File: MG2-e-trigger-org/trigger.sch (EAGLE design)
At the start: 20 parts, among them IC1 4538D, T1 BC847, T2 BC847

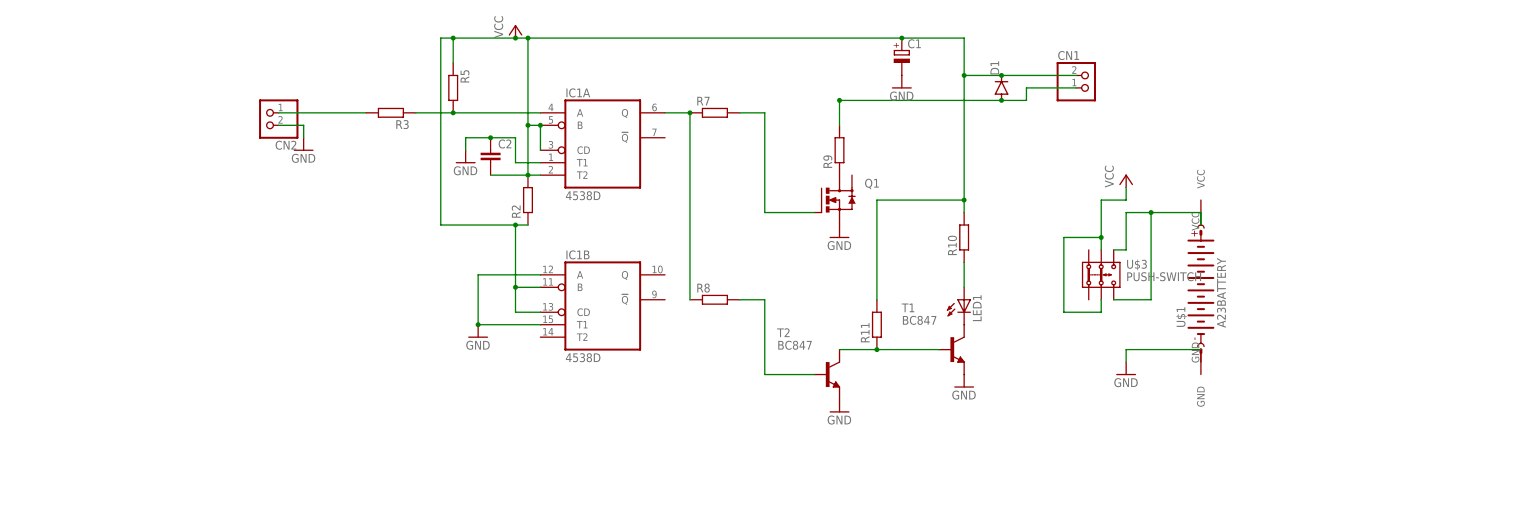
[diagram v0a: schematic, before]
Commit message: MG2 trigger
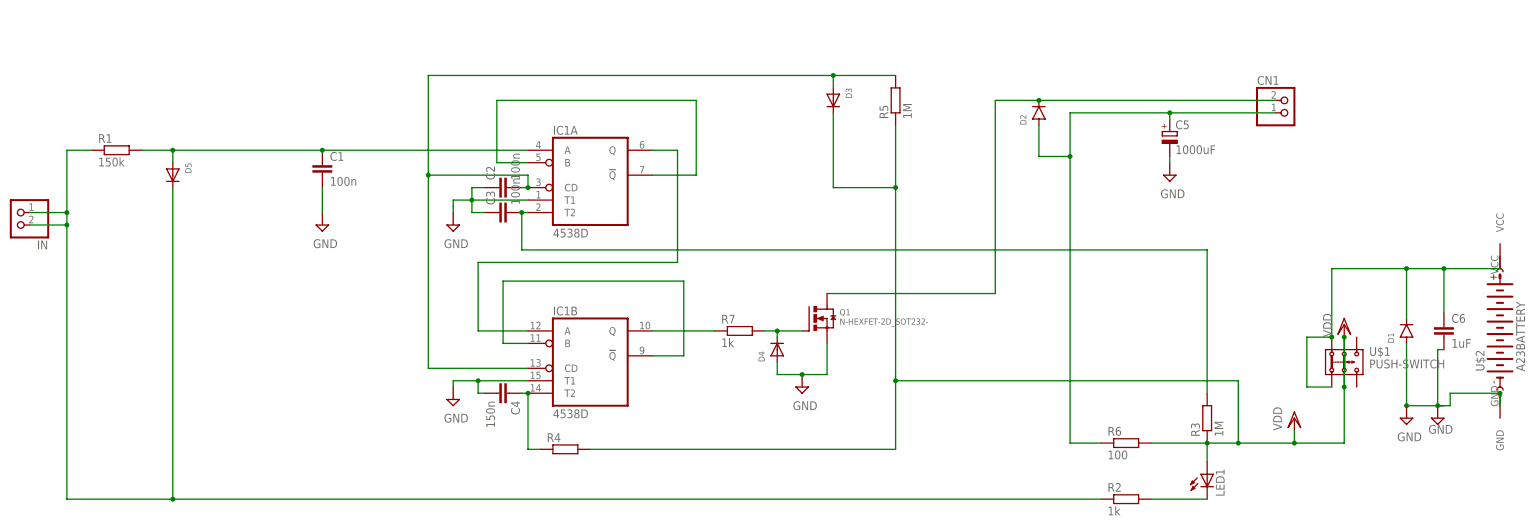
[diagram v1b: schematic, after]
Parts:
- removed CN2: (no value), adafruit:JST_2PIN-THM
- removed R10, R11: (no value), eagle-ltspice:R
- removed R8, R9: (no value), eagle-ltspice:RR1206
- removed T1, T2: BC847, nxp_60:BC847
- removed U$3: PUSH-SWITCH, zort-library:PUSH-SWITCH
- added C3: 100n, eagle-ltspice:C
- added C4: 150n, eagle-ltspice:C
- added C5: 1000uF, rcl:CPOL-EUE5-6
- added C6: 1uF, eagle-ltspice:CC1808
- added D2: (no value), semicon-smd-ipc:D-SMB
- added D3, D4, D5: (no value), adafruit:DIODESOD-123
- added IN: (no value), adafruit:JST_2PIN-THM
- added R1: 150k, eagle-ltspice:RR1206
- added R4: (no value), eagle-ltspice:RR1206
- added R6: 100, eagle-ltspice:RR2512
- added U$2: A23BATTERY, zort-library:A23BATTERY
- C1: value (none) -> 100n; device rcl:CPOL-EUE5-6 -> eagle-ltspice:C
- C2: value (none) -> 100n
- D1: device diode:DIODE-DO214AC -> semicon-smd-ipc:D-SMB
- Q1: value (none) -> N-HEXFET-2D_SOT232-; device m-pad-2.1:MOSFET_N_SOT223 -> transistor-power:N-HEXFET-2D_SOT232-
- R2, R7: value (none) -> 1k
- R3, R5: value (none) -> 1M
- U$1: value A23BATTERY -> PUSH-SWITCH; device zort-library:A23BATTERY -> zort-library:PUSH-SWITCH
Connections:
- removed net VCC: C1.+, C2.2, CN1.1, D1.C, IC1A.B, IC1A.CD, IC1A.T2, IC1B.B, IC1B.CD, R10.2, R11.2, R2.1, R2.2, R5.1, U$3.2.1, U$3.2.2
- new net N$10: C2.2, D3.A, IC1A.CD, IC1B.CD, R5.2
- new net N$13: CN1.1, D2.C, Q1.D
- new net N$14: C5.+, CN1.2, D2.A, R6.1
- new net VDD: D3.C, LED1.A, R3.1, R4.2, R5.1, R6.2, U$1.2.1, U$1.2.2
- net GND: now also C1.2, C3.1, C4.2, C5.-, C6.2, D1.A, D4.A, U$2.GND; no longer C1.-, CN2.1, IC1B.A, T1.E, T2.E, U$1.GND
- net N$1: now also C6.1, D1.C, U$1.1.1, U$1.1.2, U$2.VCC; no longer LED1.C, T1.C
- net N$11: now also IC1B.Q, R7.1; no longer U$1.VCC, U$3.3.1, U$3.3.2
- net N$12: now also D4.C
- net N$2: now also IC1B.!Q, IC1B.B; no longer CN2.2, R3.2
- net N$3: now also IC1A.!Q, IC1A.B; no longer IC1A.A, R3.1, R5.2
- net N$4: now also IC1B.A; no longer R7.1, R8.1
- net N$5: now also D5.C, IN.1, IN.2, R1.1, R2.1; no longer Q1.D, R9.1
- net N$6: now also C1.1, D5.A, IC1A.A, R1.2; no longer R8.2, T2.B
- net N$7: now also LED1.C, R2.2; no longer CN1.2, D1.A, R9.2
- net N$8: now also C4.1, IC1B.T2, R4.1; no longer R11.1, T1.B, T2.C
- net N$9: now also C3.2, IC1A.T2, R3.2; no longer LED1.A, R10.1
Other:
- moved on the sheet: C2, CN1, D1, IC1A, IC1B, LED1, R2, R3, R5, R7
